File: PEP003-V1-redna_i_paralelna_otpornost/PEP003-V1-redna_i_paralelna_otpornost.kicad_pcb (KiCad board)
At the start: 2 copper layers, 90 x 45 mm, 41 parts, among them J1 Screw_Terminal_01x02

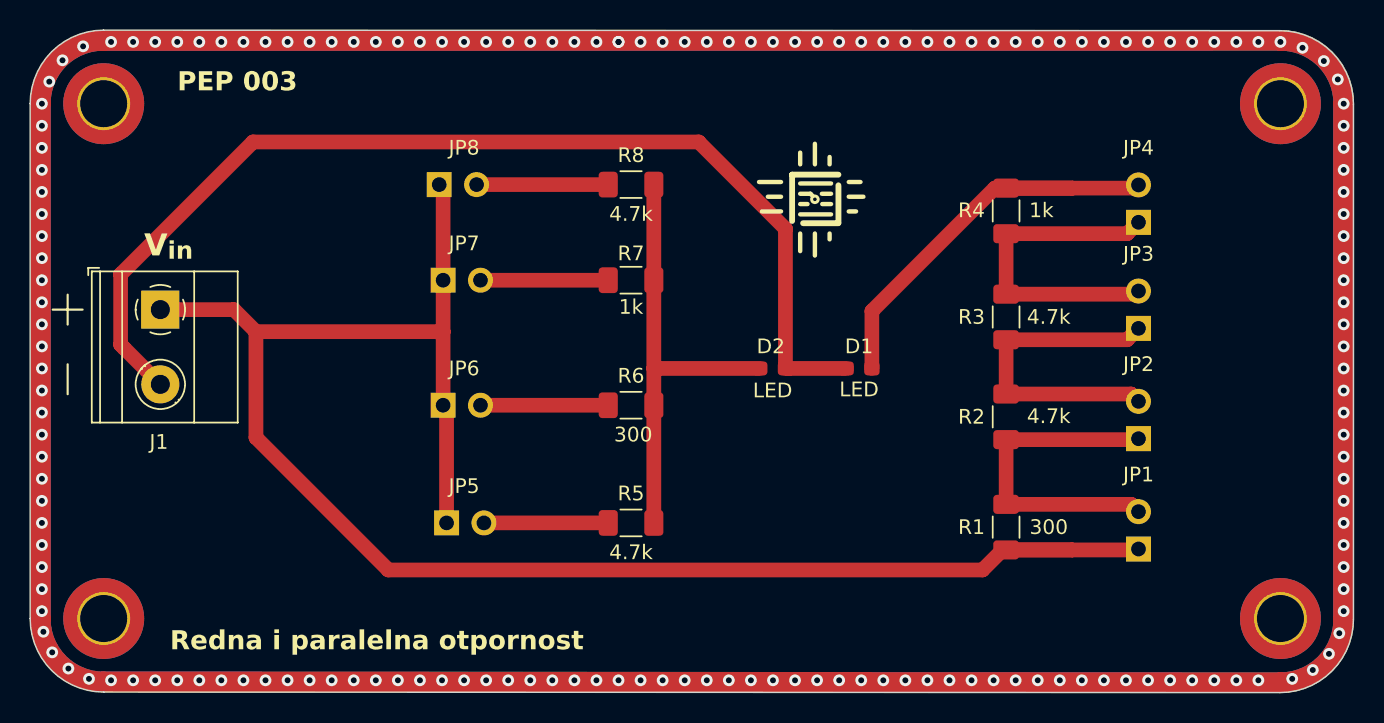
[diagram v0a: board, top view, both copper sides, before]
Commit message: Update 1,2,3,4,5,7, lib.
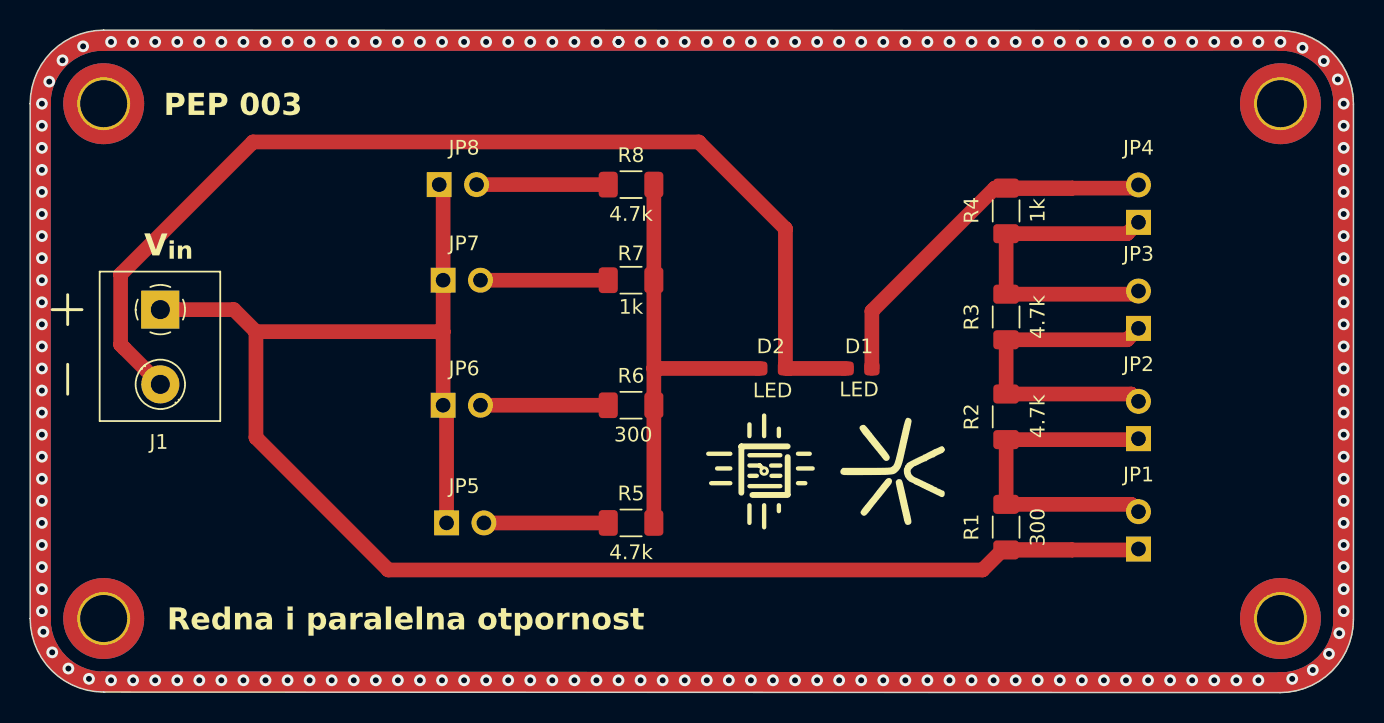
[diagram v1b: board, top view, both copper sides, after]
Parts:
- removed the G*** at (157.3, 72.5)
- added G***: LOGO, PEP_library:petnica_logo, F.Cu at (162.7, 91.0)
- moved REF** 18.8 mm to (153.9, 91.0)
- moved REF** 5.46 mm to (139.1, 99.6)
- moved REF** 5.46 mm to (140.8, 99.6)
- moved REF** 4.48 mm to (139.0, 90.1)
- moved REF** 4.48 mm to (140.8, 90.1)
- moved REF** 4.47 mm to (139.0, 68.5)
- moved REF** 4.47 mm to (140.8, 68.5)
- moved REF** 3.91 mm to (140.8, 78.1)
- moved REF** 3.91 mm to (139.0, 78.1)
- moved REF** 2.35 mm to (177.0, 72.8)
- moved REF** 2.35 mm to (167.9, 90.1)
- moved REF** 2.35 mm to (177.0, 80.5)
- moved REF** 2.35 mm to (167.9, 75.3)
- moved REF** 2.35 mm to (167.9, 68.6)
- moved REF** 2.35 mm to (167.9, 82.6)
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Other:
- board text added: "D1"
- board text added: "D2"
- board text added: "JP1"
- board text added: "JP2"
- board text added: "JP3"
- board text added: "JP4"
- board text added: "JP5"
- board text added: "JP6"
- board text added: "JP7"
- board text added: "JP8"
- board text added: "R1"
- board text added: "R2"
- board text added: "R3"
- board text added: "R4"
- board text added: "R5"
- board text added: "R6"
- board text added: "R7"
- board text added: "R8"
